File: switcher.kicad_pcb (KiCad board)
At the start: 2 copper layers, 137.5 x 100 mm, 67 parts, among them K1 RELAY, P1 CONN_01X02, P10 CONN_01X04, P11 CONN_01X04, P12 CONN_01X04, P13 CONN_01X04, P2 CONN_01X02, P3 CONN_01X04, P4 CONN_01X04, P5 CONN_01X04, P6 CONN_01X02, P7 CONN_01X04, P8 CONN_01X04, P9 BDM, Q1 BC237, SW1 RESET, SW2 SP3T, T1 TRANSFO, U1 MC9S08SH8, U10 4N25, U11 4N25, U12 4N25, U13 4N25, U14 4N25, U2 78L05, U3 4N25, U4 4N25, U5 4N25, U6 4N25, U7 4N25, U8 4N25, U9 4N25

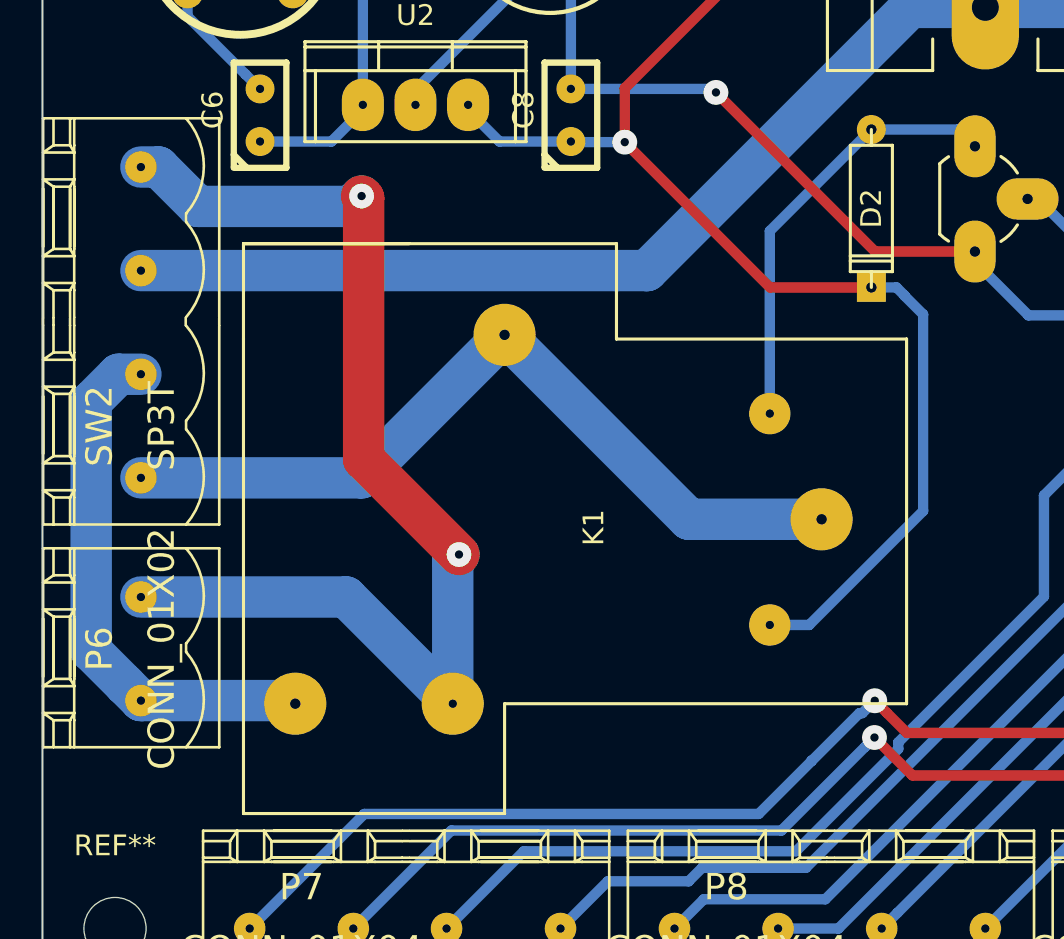
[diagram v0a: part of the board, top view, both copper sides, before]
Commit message: di vueltas el relay
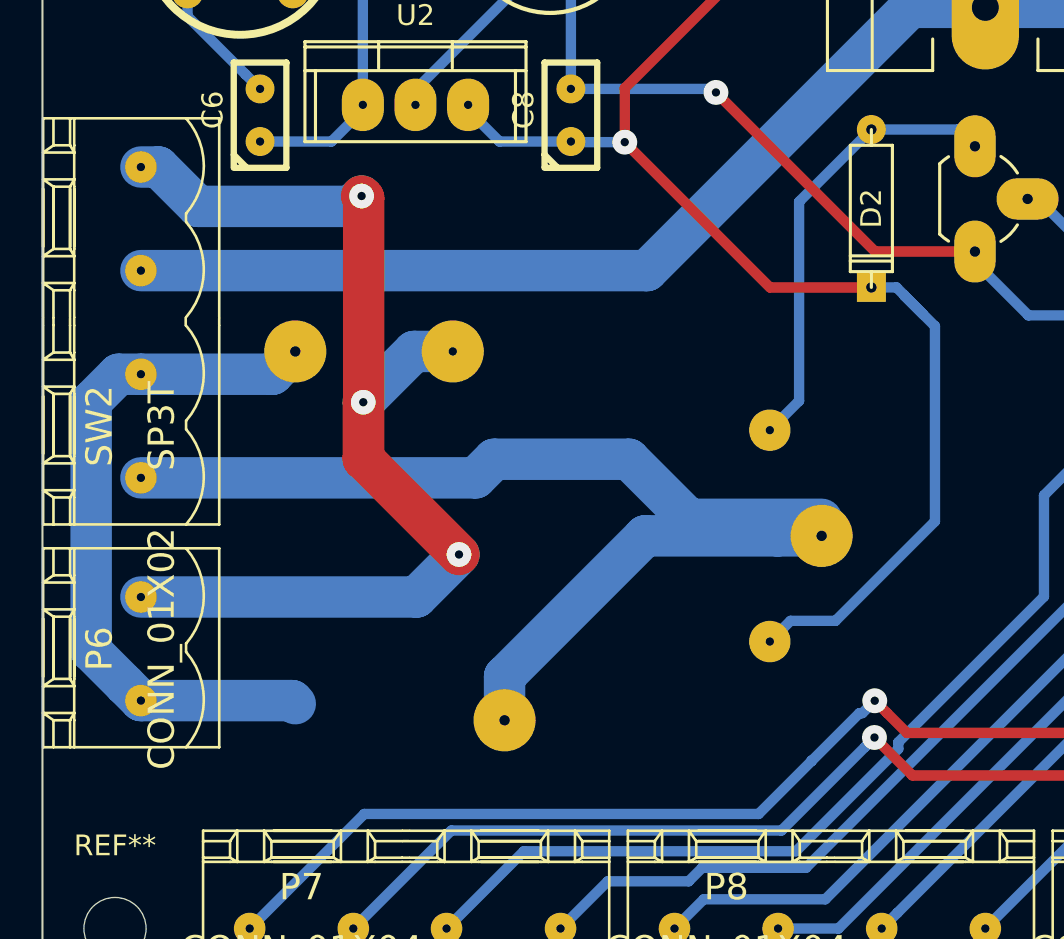
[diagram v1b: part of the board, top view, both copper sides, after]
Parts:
- K1: moved to B.Cu
- turned K1 to 270 degrees
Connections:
- K1 pad 4: /vreg -> Net-(D2-Pad1)
- K1 pad 5: Net-(D2-Pad1) -> /vreg
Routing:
- net /C: track 39.4 -> 54.7 mm
- net /NC: track 25.9 -> 33.8 mm
- net /vreg: track 255.9 -> 258.6 mm
- net Net-(D2-Pad1): track 21.1 -> 21.9 mm
- net /NA: track 55.4 -> 55.2 mm, vias 2 -> 3
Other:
- net class Default: trace_width 0.5 -> 2
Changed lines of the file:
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@@
     (links 125)
     (no_connects 0)
-    (area 74.449999 29.949999 212.050001 130.050001)
+    (area 71.361474 28.2245 217.140046 132.37626)
     (thickness 1.6)
     (drawings 4)
-    (tracks 668)
+    (tracks 681)
     (zones 0)
     (modules 67)
@@
   )
   (setup
-    (last_trace_width 0.5)
+    (last_trace_width 2)
     (trace_clearance 0.35)
     (zone_clearance 0.508)
@@
     (mod_text_size 1 1)
     (mod_text_width 0.15)
-    (pad_size 3 3)
-    (pad_drill 0.5)
+    (pad_size 2 2)
+    (pad_drill 0.4)
     (pad_to_mask_clearance 0)
     (aux_axis_origin 0 0)
@@
   (net_class Default "This is the default net class."
     (clearance 0.35)
-    (trace_width 0.5)
+    (trace_width 2)
     (via_dia 1.2)
     (via_drill 0.4)
@@
       (xy 5.87248 -0.74168) (xy 6.01472 -1.016) (xy 6.01472 -1.016)) (layer B.Cu) (width 0.00254))
   )
-  (module locales:RELAY-HJQ-15F (layer F.Cu)
-    (at 100.2 106.9 90)
-    (fp_text reference K1 (at 0 0.9 90) (layer F.SilkS)
-      (effects (font (size 1 1) (thickness 0.15)))
-    )
-    (fp_text value RELAY (at 0 -0.8 90) (layer F.Fab)
-      (effects (font (size 1 1) (thickness 0.15)))
-    )
-    (fp_line (start 9.1 2) (end 9.1 16) (layer F.SilkS) (width 0.15))
-    (fp_line (start 13.7 -16) (end 13.7 2) (layer F.SilkS) (width 0.15))
-    (fp_line (start 13.7 2) (end 9.1 2) (layer F.SilkS) (width 0.15))
-    (fp_line (start 13.7 -16) (end 9.1 -16) (layer F.SilkS) (width 0.15))
-    (fp_line (start 9.1 16) (end -8.5 16) (layer F.SilkS) (width 0.15))
-    (fp_line (start 13.7 -8) (end 13.7 -16) (layer F.SilkS) (width 0.15))
-    (fp_line (start -8.5 -3.4) (end -8.5 16) (layer F.SilkS) (width 0.15))
-    (fp_line (start -13.8 -3.4) (end -13.8 -16) (layer F.SilkS) (width 0.15))
-    (fp_line (start -13.8 -16) (end -8.5 -16) (layer F.SilkS) (width 0.15))
-    (fp_line (start -13.8 -3.4) (end -8.5 -3.4) (layer F.SilkS) (width 0.15))
-    (fp_line (start -8.5 -16) (end 9.1 -16) (layer F.SilkS) (width 0.15))
-    (pad 1 thru_hole circle (at -8.5 -13.5 90) (size 3 3) (drill 0.5) (layers *.Cu *.Mask F.SilkS)
+  (module locales:RELAY-HJQ-15F (layer B.Cu)
+    (at 100.2 106.9 270)
+    (fp_text reference K1 (at 0 -0.9 270) (layer B.SilkS)
+      (effects (font (size 1 1) (thickness 0.15)) (justify mirror))
+    )
+    (fp_text value RELAY (at 0 0.8 270) (layer B.Fab)
+      (effects (font (size 1 1) (thickness 0.15)) (justify mirror))
+    )
+    (fp_line (start 9.1 -2) (end 9.1 -16) (layer B.SilkS) (width 0.15))
+    (fp_line (start 13.7 16) (end 13.7 -2) (layer B.SilkS) (width 0.15))
+    (fp_line (start 13.7 -2) (end 9.1 -2) (layer B.SilkS) (width 0.15))
+    (fp_line (start 13.7 16) (end 9.1 16) (layer B.SilkS) (width 0.15))
+    (fp_line (start 9.1 -16) (end -8.5 -16) (layer B.SilkS) (width 0.15))
+    (fp_line (start 13.7 8) (end 13.7 16) (layer B.SilkS) (width 0.15))
+    (fp_line (start -8.5 3.4) (end -8.5 -16) (layer B.SilkS) (width 0.15))
+    (fp_line (start -13.8 3.4) (end -13.8 16) (layer B.SilkS) (width 0.15))
+    (fp_line (start -13.8 16) (end -8.5 16) (layer B.SilkS) (width 0.15))
+    (fp_line (start -13.8 3.4) (end -8.5 3.4) (layer B.SilkS) (width 0.15))
+    (fp_line (start -8.5 16) (end 9.1 16) (layer B.SilkS) (width 0.15))
+    (pad 1 thru_hole circle (at -8.5 13.5 270) (size 3 3) (drill 0.5) (layers *.Cu *.Mask B.SilkS)
       (net 10 /NC))
-    (pad 2 thru_hole circle (at -8.5 -5.9 90) (size 3 3) (drill 0.4) (layers *.Cu *.Mask F.SilkS)
+    (pad 2 thru_hole circle (at -8.5 5.9 270) (size 3 3) (drill 0.4) (layers *.Cu *.Mask B.SilkS)
       (net 8 /NA))
-    (pad 3 thru_hole circle (at 9.3 -3.4 90) (size 3 3) (drill 0.5) (layers *.Cu *.Mask F.SilkS)
+    (pad 3 thru_hole circle (at 9.3 3.4 270) (size 3 3) (drill 0.5) (layers *.Cu *.Mask B.SilkS)
       (net 9 /C))
-    (pad 4 thru_hole circle (at -4.7 9.4 90) (size 2 2) (drill 0.4) (layers *.Cu *.Mask F.SilkS)
-      (net 2 /vreg))
-    (pad 5 thru_hole circle (at 5.5 9.4 90) (size 2 2) (drill 0.4) (layers *.Cu *.Mask F.SilkS)
+    (pad 4 thru_hole circle (at -4.7 -9.4 270) (size 2 2) (drill 0.4) (layers *.Cu *.Mask B.SilkS)
       (net 1 "Net-(D2-Pad1)"))
-    (pad 6 thru_hole circle (at 0.4 11.9 90) (size 3 3) (drill 0.5) (layers *.Cu *.Mask F.SilkS)
+    (pad 5 thru_hole circle (at 5.5 -9.4 270) (size 2 2) (drill 0.4) (layers *.Cu *.Mask B.SilkS)
+      (net 2 /vreg))
+    (pad 6 thru_hole circle (at 0.4 -11.9 270) (size 3 3) (drill 0.5) (layers *.Cu *.Mask B.SilkS)
       (net 9 /C))
   )
@@
   (gr_line (start 74.5 130) (end 74.5 30) (angle 90) (layer Edge.Cuts) (width 0.1))
   (gr_line (start 74.5 130) (end 212 130) (angle 90) (layer Edge.Cuts) (width 0.1))
+  (segment (start 111.013284 100.786716) (end 111.013284 91.176716) (width 0.5) (layer B.Cu) (net 1))
+  (segment (start 111.013284 91.176716) (end 114.5 87.69) (width 0.5) (layer B.Cu) (net 1))
+  (segment (start 109.6 102.2) (end 111.013284 100.786716) (width 0.5) (layer B.Cu) (net 1))
   (segment (start 114.5 87.69) (end 118.69 87.69) (width 0.5) (layer B.Cu) (net 1))
   (segment (start 118.69 87.69) (end 119.5 88.5) (width 0.5) (layer B.Cu) (net 1))
-  (segment (start 109.6 101.4) (end 109.6 92.59) (width 0.5) (layer B.Cu) (net 1))
-  (segment (start 109.6 92.59) (end 114.5 87.69) (width 0.5) (layer B.Cu) (net 1))
-  (segment (start 109.6 111.6) (end 111.5 111.6) (width 0.5) (layer B.Cu) (net 2))
-  (segment (start 111.5 111.6) (end 117 106.1) (width 0.5) (layer B.Cu) (net 2))
+  (segment (start 109.6 112.4) (end 110.599999 111.400001) (width 0.5) (layer B.Cu) (net 2))
+  (segment (start 110.599999 111.400001) (end 112.769999 111.400001) (width 0.5) (layer B.Cu) (net 2))
+  (segment (start 112.769999 111.400001) (end 117.57 106.6) (width 0.5) (layer B.Cu) (net 2))
+  (segment (start 117.57 97.1815) (end 116.1 95.7115) (width 0.5) (layer B.Cu) (net 2))
+  (segment (start 117.57 106.6) (end 117.57 97.1815) (width 0.5) (layer B.Cu) (net 2))
   (segment (start 114.5 95.31) (end 115.71 95.31) (width 0.5) (layer B.Cu) (net 2))
   (segment (start 116.1 95.7) (end 116.1 95.7115) (width 0.5) (layer B.Cu) (net 2))
   (segment (start 115.71 95.31) (end 116.1 95.7) (width 0.5) (layer B.Cu) (net 2))
   (segment (start 117 96.6115) (end 116.1 95.7115) (width 0.5) (layer B.Cu) (net 2))
-  (segment (start 117 106.1) (end 117 96.6115) (width 0.5) (layer B.Cu) (net 2))
   (segment (start 102.6 85.7) (end 111.8 76.5) (width 0.5) (layer F.Cu) (net 2))
   (segment (start 111.8 76.5) (end 115.5 76.5) (width 0.5) (layer F.Cu) (net 2))
@@
   (segment (start 103.25 45.5) (end 118.704 45.5) (width 2) (layer B.Cu) (net 7))
   (segment (start 118.704 45.5) (end 120 44.204) (width 2) (layer B.Cu) (net 7))
+  (segment (start 89.98 100.85) (end 89.98 103.58) (width 2) (layer F.Cu) (net 8))
+  (segment (start 89.98 103.58) (end 90 103.6) (width 2) (layer F.Cu) (net 8))
+  (segment (start 94.3 98.4) (end 92.43 98.4) (width 2) (layer B.Cu) (net 8))
+  (segment (start 92.43 98.4) (end 89.98 100.85) (width 2) (layer B.Cu) (net 8))
+  (via (at 89.98 100.85) (size 1.2) (drill 0.4) (layers F.Cu B.Cu) (net 8))
+  (segment (start 79.25 110.25) (end 92.55 110.25) (width 2) (layer B.Cu) (net 8))
+  (segment (start 92.55 110.25) (end 94.6 108.2) (width 2) (layer B.Cu) (net 8))
   (segment (start 79.25 89.5) (end 80.1 89.5) (width 2) (layer B.Cu) (net 8))
-  (segment (start 94.3 108.5) (end 94.3 115.4) (width 2) (layer B.Cu) (net 8))
-  (segment (start 94.6 108.2) (end 94.3 108.5) (width 2) (layer B.Cu) (net 8))
   (via (at 94.6 108.2) (size 1.2) (drill 0.4) (layers F.Cu B.Cu) (net 8))
   (segment (start 90 103.6) (end 94.6 108.2) (width 2) (layer F.Cu) (net 8))
@@
   (segment (start 82 91.4) (end 89.4 91.4) (width 2) (layer B.Cu) (net 8))
   (segment (start 80.1 89.5) (end 82 91.4) (width 2) (layer B.Cu) (net 8))
-  (segment (start 79.25 110.25) (end 89.15 110.25) (width 2) (layer B.Cu) (net 8))
-  (segment (start 89.15 110.25) (end 94.3 115.4) (width 2) (layer B.Cu) (net 8))
+  (segment (start 96.8 116.2) (end 96.8 114.07868) (width 2) (layer B.Cu) (net 9))
+  (segment (start 96.8 114.07868) (end 103.57868 107.3) (width 2) (layer B.Cu) (net 9))
+  (segment (start 103.57868 107.3) (end 109.97868 107.3) (width 2) (layer B.Cu) (net 9))
+  (segment (start 109.97868 107.3) (end 112.1 107.3) (width 2) (layer B.Cu) (net 9))
+  (segment (start 105.7 106.5) (end 102.80291 103.60291) (width 2) (layer B.Cu) (net 9))
+  (segment (start 96.29709 103.60291) (end 102.80291 103.60291) (width 2) (layer B.Cu) (net 9))
+  (segment (start 95.4 104.5) (end 96.29709 103.60291) (width 2) (layer B.Cu) (net 9))
+  (segment (start 79.25 104.5) (end 95.4 104.5) (width 2) (layer B.Cu) (net 9))
   (segment (start 112.1 106.5) (end 105.7 106.5) (width 2) (layer B.Cu) (net 9))
-  (segment (start 105.7 106.5) (end 96.8 97.6) (width 2) (layer B.Cu) (net 9))
-  (segment (start 79.25 104.5) (end 89.9 104.5) (width 2) (layer B.Cu) (net 9))
-  (segment (start 89.9 104.5) (end 96.8 97.6) (width 2) (layer B.Cu) (net 9))
+  (segment (start 79.25 99.5) (end 85.6 99.5) (width 2) (layer B.Cu) (net 10))
+  (segment (start 85.6 99.5) (end 86.7 98.4) (width 2) (layer B.Cu) (net 10))
   (segment (start 79.25 99.5) (end 78.17237 99.5) (width 2) (layer B.Cu) (net 10))
   (segment (start 78.17237 99.5) (end 76.84999 100.82238) (width 2) (layer B.Cu) (net 10))
